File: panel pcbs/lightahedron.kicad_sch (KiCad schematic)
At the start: 60 parts, among them J1 CONN, M1 Magnet 5x2mm, M2 Magnet 5x2mm, M3 Magnet 5x2mm

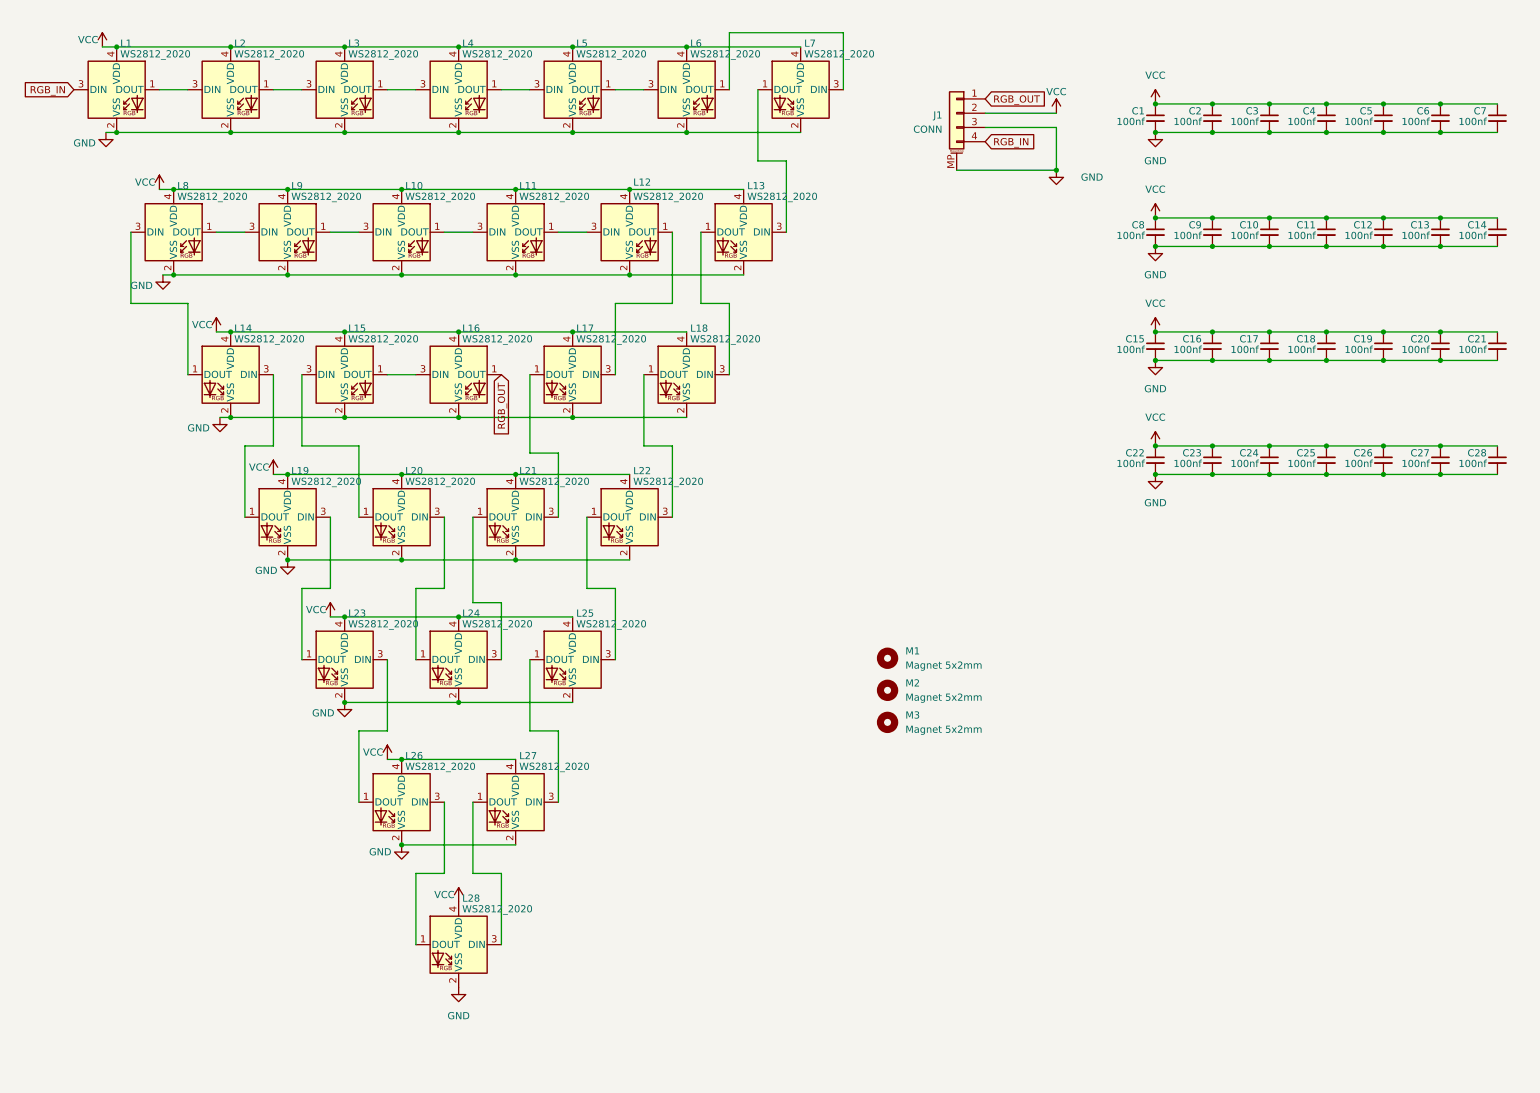
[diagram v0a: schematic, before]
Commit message: cleanup, work on pcbs, finish frame, add render
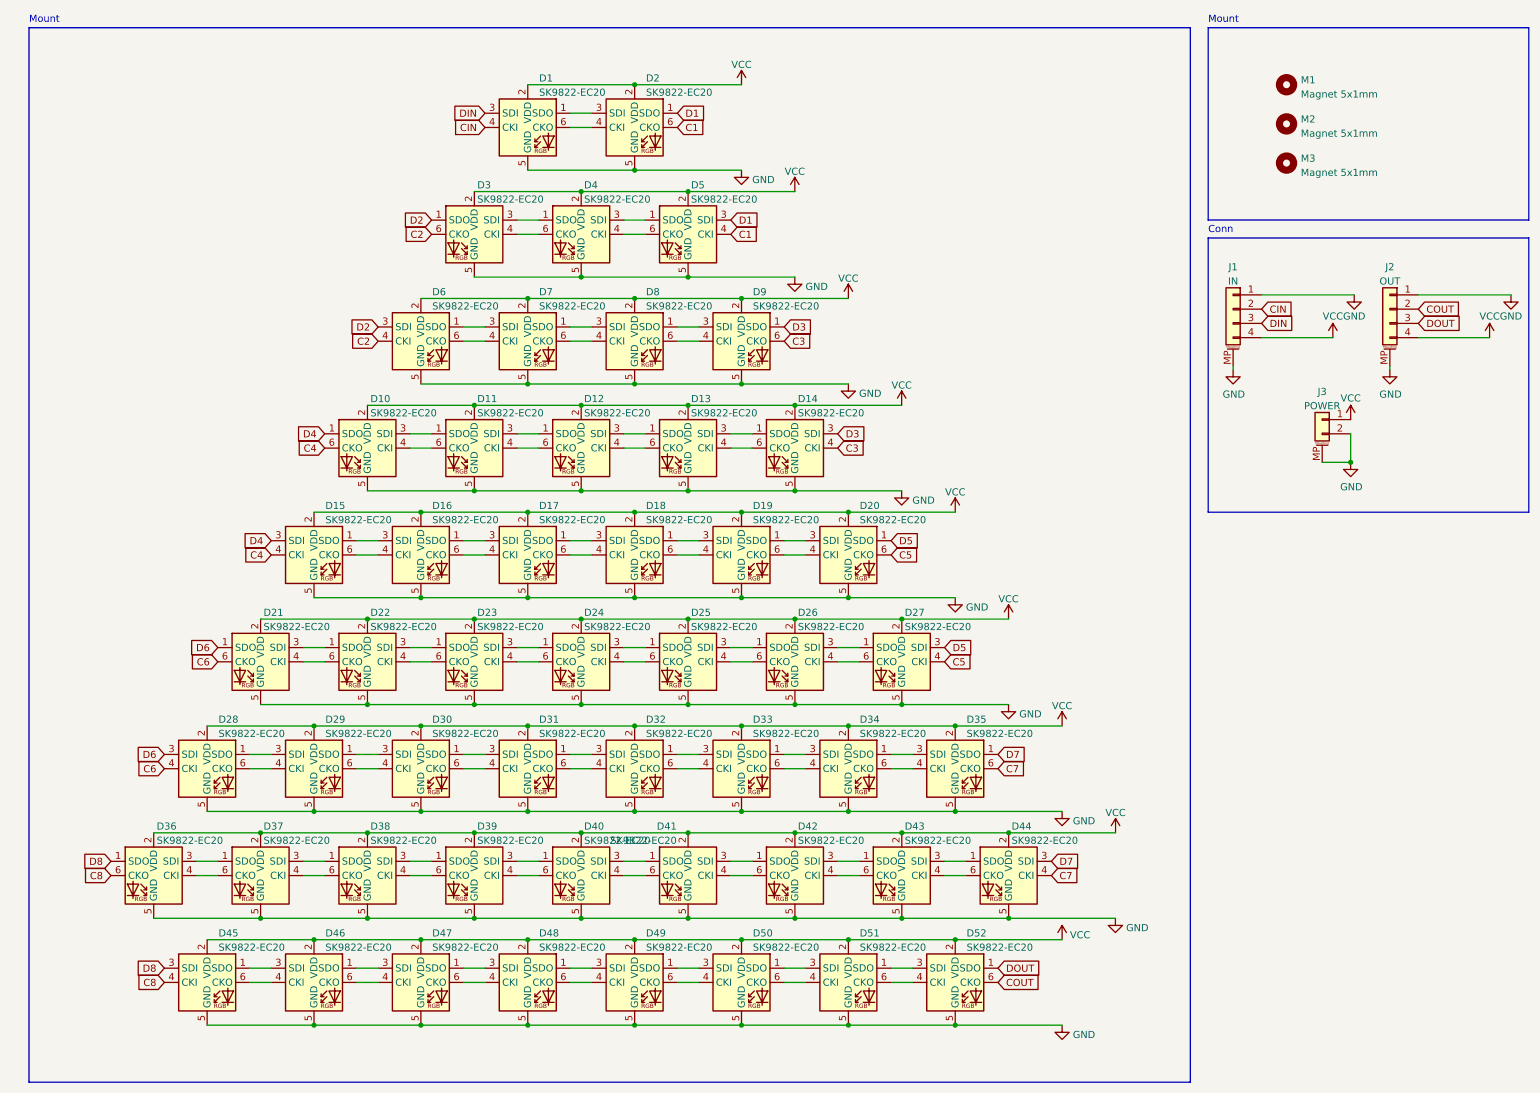
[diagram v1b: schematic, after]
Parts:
- removed C1, C10, C11, C12, C13, C14, C15, C16, C17, C18, C19, C2, C20, C21, C22, C23, C24, C25, C26, C27, C28, C3, C4, C5, C6, C7, C8, C9: 100nf, Capacitor_SMD:C_0402_1005Metric, symbol Device:C_Small
- removed L1, L10, L11, L12, L13, L14, L15, L16, L17, L18, L19, L2, L20, L21, L22, L23, L24, L25, L26, L27, L28, L3, L4, L5, L6, L7, L8, L9: WS2812_2020, marbastlib-various:LED_WS2812_2020, symbol marbastlib-various:WS2812_2020
- added D1, D10, D11, D12, D13, D14, D15, D16, D17, D18, D19, D2, D20, D21, D22, D23, D24, D25, D26, D27, D28, D29, D3, D30, D31, D32, D33, D34, D35, D36, D37, D38, D39, D4, D40, D41, D42, D43, D44, D45, D46, D47, D48, D49, D5, D50, D51, D52, D6, D7, D8, D9: SK9822-EC20, custom:sk9822-2020, symbol custom:SK9822-EC20
- added J2: OUT, Connector_JST:JST_SH_SM04B-SRSS-TB_1x04-1MP_P1.00mm_Horizontal, symbol Connector_Generic_MountingPin:Conn_01x04_MountingPin
- added J3: POWER, Connector_JST:JST_SH_SM02B-SRSS-TB_1x02-1MP_P1.00mm_Horizontal, symbol Connector_Generic_MountingPin:Conn_01x02_MountingPin
- J1: value CONN -> IN
- M1, M2, M3: value Magnet 5x2mm -> Magnet 5x1mm; footprint magnets:Magnet_D5mm_L2mm -> custom:Magnet_D5mm_L2mm
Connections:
- net RGB_IN is gone; now on net VCC: J1.4 (Pin_4)
- net RGB_OUT is gone; now on net GND: J1.1 (Pin_1)
- net GND: now also D1.5 (GND), D10.5 (GND), D11.5 (GND), D12.5 (GND), D13.5 (GND), D14.5 (GND), D15.5 (GND), D16.5 (GND), D17.5 (GND), D18.5 (GND), D19.5 (GND), D2.5 (GND), D20.5 (GND), D21.5 (GND), D22.5 (GND), D23.5 (GND), D24.5 (GND), D25.5 (GND), D26.5 (GND), D27.5 (GND), D28.5 (GND), D29.5 (GND), D3.5 (GND), D30.5 (GND), D31.5 (GND), D32.5 (GND), D33.5 (GND), D34.5 (GND), D35.5 (GND), D36.5 (GND), D37.5 (GND), D38.5 (GND), D39.5 (GND), D4.5 (GND), D40.5 (GND), D41.5 (GND), D42.5 (GND), D43.5 (GND), D44.5 (GND), D45.5 (GND), D46.5 (GND), D47.5 (GND), D48.5 (GND), D49.5 (GND), D5.5 (GND), D50.5 (GND), D51.5 (GND), D52.5 (GND), D6.5 (GND), D7.5 (GND), D8.5 (GND), D9.5 (GND), J2.1 (Pin_1), J2.MP (MountPin), J3.2 (Pin_2), J3.MP (MountPin); no longer J1.3 (Pin_3)
- net VCC: now also D1.2 (VDD), D10.2 (VDD), D11.2 (VDD), D12.2 (VDD), D13.2 (VDD), D14.2 (VDD), D15.2 (VDD), D16.2 (VDD), D17.2 (VDD), D18.2 (VDD), D19.2 (VDD), D2.2 (VDD), D20.2 (VDD), D21.2 (VDD), D22.2 (VDD), D23.2 (VDD), D24.2 (VDD), D25.2 (VDD), D26.2 (VDD), D27.2 (VDD), D28.2 (VDD), D29.2 (VDD), D3.2 (VDD), D30.2 (VDD), D31.2 (VDD), D32.2 (VDD), D33.2 (VDD), D34.2 (VDD), D35.2 (VDD), D36.2 (VDD), D37.2 (VDD), D38.2 (VDD), D39.2 (VDD), D4.2 (VDD), D40.2 (VDD), D41.2 (VDD), D42.2 (VDD), D43.2 (VDD), D44.2 (VDD), D45.2 (VDD), D46.2 (VDD), D47.2 (VDD), D48.2 (VDD), D49.2 (VDD), D5.2 (VDD), D50.2 (VDD), D51.2 (VDD), D52.2 (VDD), D6.2 (VDD), D7.2 (VDD), D8.2 (VDD), D9.2 (VDD), J2.4 (Pin_4), J3.1 (Pin_1); no longer J1.2 (Pin_2)
- new net: D51.1 (SDO), D52.3 (SDI)
- new net: D51.6 (CKO), D52.4 (CKI)
- new net: D47.1 (SDO), D48.3 (SDI)
- new net: D46.1 (SDO), D47.3 (SDI)
- new net: D46.6 (CKO), D47.4 (CKI)
- new net: D47.6 (CKO), D48.4 (CKI)
- new net: D3.3 (SDI), D4.1 (SDO)
- new net: D3.4 (CKI), D4.6 (CKO)
- new net: D50.1 (SDO), D51.3 (SDI)
- new net: D49.1 (SDO), D50.3 (SDI)
- new net: D49.6 (CKO), D50.4 (CKI)
- new net: D50.6 (CKO), D51.4 (CKI)
- new net: D32.1 (SDO), D33.3 (SDI)
- new net: D31.1 (SDO), D32.3 (SDI)
- new net: D31.6 (CKO), D32.4 (CKI)
- new net: D32.6 (CKO), D33.4 (CKI)
- new net: D4.3 (SDI), D5.1 (SDO)
- new net: D4.4 (CKI), D5.6 (CKO)
- new net: D1.1 (SDO), D2.3 (SDI)
- new net: D1.6 (CKO), D2.4 (CKI)
- new net: D10.3 (SDI), D11.1 (SDO)
- new net: D11.3 (SDI), D12.1 (SDO)
- new net: D11.4 (CKI), D12.6 (CKO)
- new net: D10.4 (CKI), D11.6 (CKO)
- new net: D39.3 (SDI), D40.1 (SDO)
- new net: D40.3 (SDI), D41.1 (SDO)
- new net: D40.4 (CKI), D41.6 (CKO)
- new net: D39.4 (CKI), D40.6 (CKO)
- new net: D29.1 (SDO), D30.3 (SDI)
- new net: D28.1 (SDO), D29.3 (SDI)
- new net: D28.6 (CKO), D29.4 (CKI)
- new net: D29.6 (CKO), D30.4 (CKI)
- new net: D25.3 (SDI), D26.1 (SDO)
- new net: D26.3 (SDI), D27.1 (SDO)
- new net: D26.4 (CKI), D27.6 (CKO)
- new net: D25.4 (CKI), D26.6 (CKO)
- new net: D48.1 (SDO), D49.3 (SDI)
- new net: D48.6 (CKO), D49.4 (CKI)
- new net: D36.3 (SDI), D37.1 (SDO)
- new net: D37.3 (SDI), D38.1 (SDO)
- new net: D37.4 (CKI), D38.6 (CKO)
- new net: D36.4 (CKI), D37.6 (CKO)
- new net: D38.3 (SDI), D39.1 (SDO)
- new net: D38.4 (CKI), D39.6 (CKO)
- new net: D12.3 (SDI), D13.1 (SDO)
- new net: D13.3 (SDI), D14.1 (SDO)
- new net: D13.4 (CKI), D14.6 (CKO)
- new net: D12.4 (CKI), D13.6 (CKO)
- new net: D24.3 (SDI), D25.1 (SDO)
- new net: D24.4 (CKI), D25.6 (CKO)
- new net: D7.1 (SDO), D8.3 (SDI)
- new net: D6.1 (SDO), D7.3 (SDI)
- new net: D6.6 (CKO), D7.4 (CKI)
- new net: D7.6 (CKO), D8.4 (CKI)
- new net: D19.1 (SDO), D20.3 (SDI)
- new net: D19.6 (CKO), D20.4 (CKI)
- new net: D22.3 (SDI), D23.1 (SDO)
- new net: D23.3 (SDI), D24.1 (SDO)
- new net: D23.4 (CKI), D24.6 (CKO)
- new net: D22.4 (CKI), D23.6 (CKO)
- new net: D33.1 (SDO), D34.3 (SDI)
- new net: D33.6 (CKO), D34.4 (CKI)
- new net: D41.3 (SDI), D42.1 (SDO)
- new net: D42.3 (SDI), D43.1 (SDO)
- new net: D42.4 (CKI), D43.6 (CKO)
- new net: D41.4 (CKI), D42.6 (CKO)
- new net: D8.1 (SDO), D9.3 (SDI)
- new net: D8.6 (CKO), D9.4 (CKI)
- new net: D45.1 (SDO), D46.3 (SDI)
- new net: D45.6 (CKO), D46.4 (CKI)
- new net: D21.3 (SDI), D22.1 (SDO)
- new net: D21.4 (CKI), D22.6 (CKO)
- new net: D30.1 (SDO), D31.3 (SDI)
- new net: D30.6 (CKO), D31.4 (CKI)
- new net: D15.1 (SDO), D16.3 (SDI)
- new net: D15.6 (CKO), D16.4 (CKI)
- new net: D34.1 (SDO), D35.3 (SDI)
- new net: D34.6 (CKO), D35.4 (CKI)
- new net: D16.1 (SDO), D17.3 (SDI)
- new net: D16.6 (CKO), D17.4 (CKI)
- new net: D43.3 (SDI), D44.1 (SDO)
- new net: D43.4 (CKI), D44.6 (CKO)
- new net: D18.1 (SDO), D19.3 (SDI)
- new net: D17.1 (SDO), D18.3 (SDI)
- new net: D17.6 (CKO), D18.4 (CKI)
- new net: D18.6 (CKO), D19.4 (CKI)
- new net C1: D2.6 (CKO), D5.4 (CKI)
- new net C2: D3.6 (CKO), D6.4 (CKI)
- new net C3: D14.4 (CKI), D9.6 (CKO)
- new net C4: D10.6 (CKO), D15.4 (CKI)
- new net C5: D20.6 (CKO), D27.4 (CKI)
- new net C6: D21.6 (CKO), D28.4 (CKI)
- new net C7: D35.6 (CKO), D44.4 (CKI)
- new net C8: D36.6 (CKO), D45.4 (CKI)
- new net CIN: D1.4 (CKI), J1.2 (Pin_2)
- new net COUT: D52.6 (CKO), J2.2 (Pin_2)
- new net D1: D2.1 (SDO), D5.3 (SDI)
- new net D2: D3.1 (SDO), D6.3 (SDI)
- new net D3: D14.3 (SDI), D9.1 (SDO)
- new net D4: D10.1 (SDO), D15.3 (SDI)
- new net D5: D20.1 (SDO), D27.3 (SDI)
- new net D6: D21.1 (SDO), D28.3 (SDI)
- new net D7: D35.1 (SDO), D44.3 (SDI)
- new net D8: D36.1 (SDO), D45.3 (SDI)
- new net DIN: D1.3 (SDI), J1.3 (Pin_3)
- new net DOUT: D52.1 (SDO), J2.3 (Pin_3)
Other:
- note added: "Conn"
- note added: "Mount"
- moved on the sheet: M1, M2, M3
